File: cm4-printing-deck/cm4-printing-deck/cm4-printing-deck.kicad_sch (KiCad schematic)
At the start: 200 parts, among them J1 Micro_SD_Card, J10 KB_USB, J2 USB_C_Receptacle_USB2.0_14P, J3 Reset, J4 debug, J5 Boot pins, J6 HDMI_A, J7 USB3_A, J8 USB3_A, J9 KB_USB, K1 KEYSW, K10 KEYSW, K11 KEYSW, K12 KEYSW, K13 KEYSW, K14 KEYSW, K15 KEYSW, K16 KEYSW, K17 KEYSW, K18 KEYSW, K19 KEYSW, K2 KEYSW, K20 KEYSW, K21 KEYSW, K22 KEYSW, K23 KEYSW, K24 KEYSW, K25 KEYSW, K26 KEYSW, K27 KEYSW, K28 KEYSW, K29 KEYSW, K3 KEYSW, K30 KEYSW, K31 KEYSW, K32 KEYSW, K33 KEYSW, K34 KEYSW, K35 KEYSW, K36 KEYSW, K37 KEYSW, K38 KEYSW, K39 KEYSW, K4 KEYSW, K40 KEYSW, K41 KEYSW, K42 KEYSW, K43 KEYSW, K44 KEYSW, K45 KEYSW, K46 KEYSW, K47 KEYSW, K48 KEYSW, K49 KEYSW, K5 KEYSW, K50 KEYSW, K51 KEYSW, K52 KEYSW, K53 KEYSW, K54 KEYSW, K55 KEYSW, K56 KEYSW, K57 KEYSW, K6 KEYSW, K60 KEYSW, K61 KEYSW, K7 KEYSW, K8 KEYSW, K9 KEYSW, SW20 Power, SW62 WIFIBT_DISABLE, U1 Compute_Module_4_Connectors, U10 AP2112K-3.3, U11 W25Q128JVS, U2 RP2040, U3 RT9742GGJ5, U5 PCF85063ATL, U6 74LVC1G07, U7 74LVC1G07, U8 74LVC1G07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

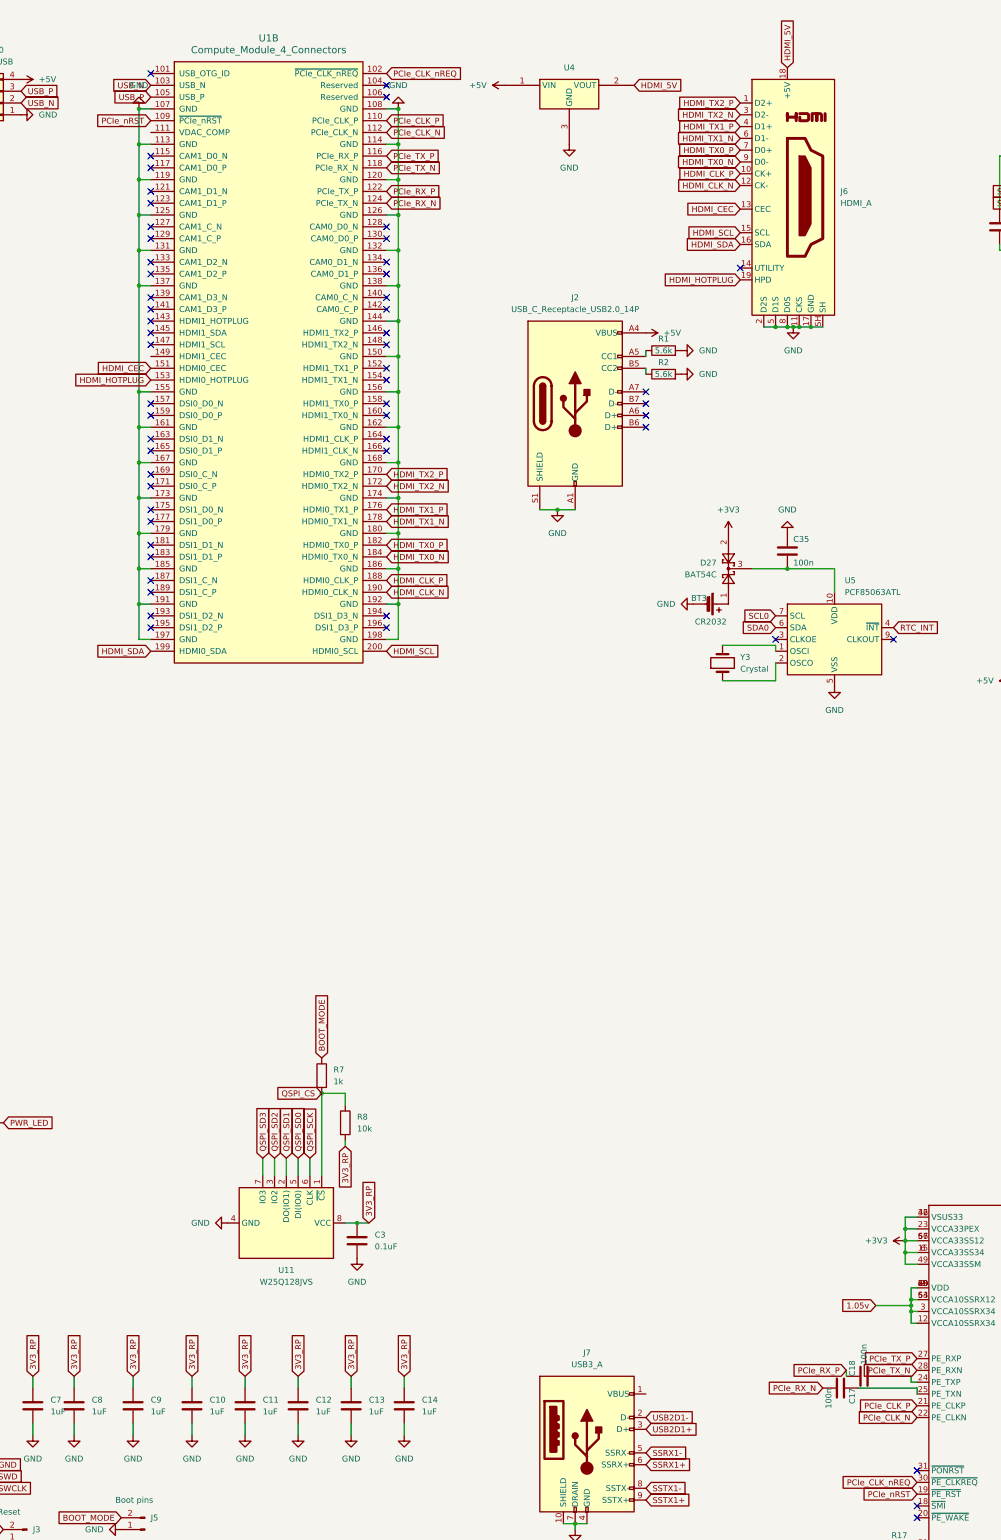
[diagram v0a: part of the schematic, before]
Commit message: minor routing and placement changes
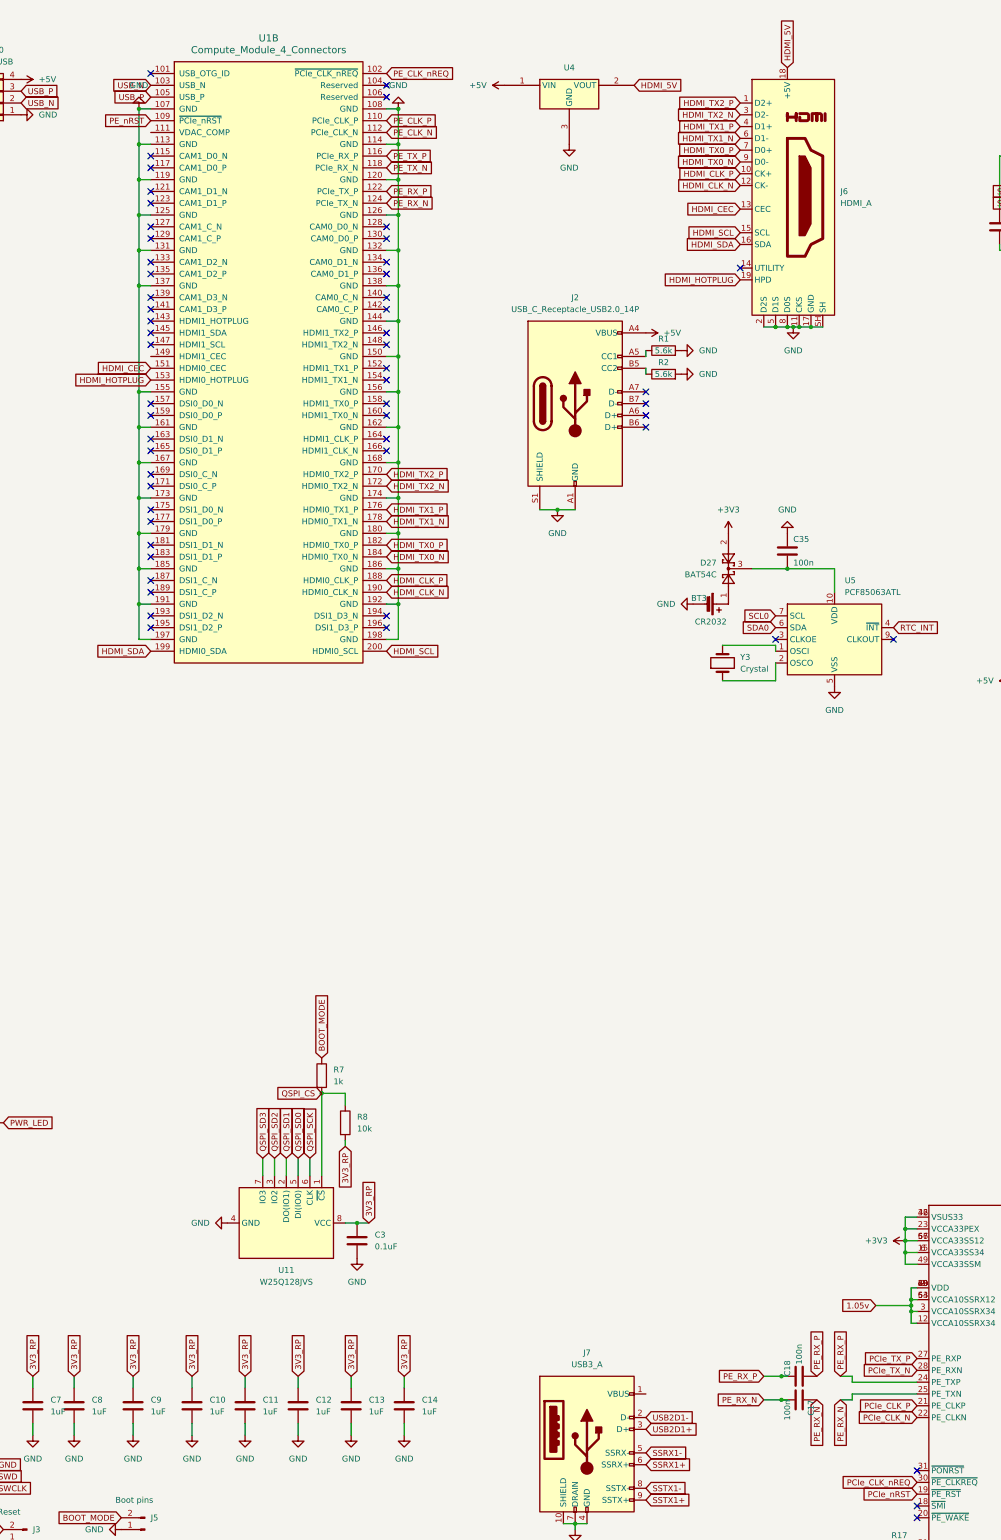
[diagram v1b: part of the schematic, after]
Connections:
- net PCIe_RX_N is gone; now on net PE_RX_N: C17.1, U1.124 (PCIe_TX_N)
- net PCIe_RX_P is gone; now on net PE_RX_P: C18.1, U1.122 (PCIe_TX_P)
- net PCIe_CLK_N: no longer U1.112 (PCIe_CLK_N)
- net PCIe_CLK_P: no longer U1.110 (PCIe_CLK_P)
- net PCIe_CLK_nREQ: no longer U1.102 (~{PCIe_CLK_nREQ})
- net PCIe_TX_N: no longer U1.118 (PCIe_RX_N)
- net PCIe_TX_P: no longer U1.116 (PCIe_RX_P)
- net PCIe_nRST: no longer U1.109 (~{PCIe_nRST})
- net PE_RX_P: now reaches C18.2, U9.24 (PE_TXP)
- net PE_RX_N: now reaches C17.2, U9.25 (PE_TXN)
- new net PE_CLK_N: U1.112 (PCIe_CLK_N)
- new net PE_CLK_P: U1.110 (PCIe_CLK_P)
- new net PE_CLK_nREQ: U1.102 (~{PCIe_CLK_nREQ})
- new net PE_TX_N: U1.118 (PCIe_RX_N)
- new net PE_TX_P: U1.116 (PCIe_RX_P)
- new net PE_nRST: U1.109 (~{PCIe_nRST})
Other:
- moved on the sheet: C17, C18

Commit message: cm4-printing-deck: added fpc connectors for dsi panel
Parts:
- added C19, C20, C21: 0.1uF 10V, Capacitor_SMD:C_0402_1005Metric, symbol Device:C
- added C22: 22uF 6.3V, Capacitor_SMD:C_0402_1005Metric, symbol Device:C
- added C23, C24, C25, C27: 0.1uF 6.3V, Capacitor_SMD:C_0402_1005Metric, symbol Device:C
- added C26: 0.1uF 6V3, Capacitor_SMD:C_0603_1608Metric, symbol Device:C
- added C4: 22uF 10V, Capacitor_SMD:C_0402_1005Metric, symbol Device:C
- added J11: 3-2328724-1, moth:3-2328724-1, symbol cm4-panel-jdi-lt070me05000-rescue:3-2328724-1-Connector
- added J12: MOLEX_503480-0600, moth:screen_conn_2_nexus, symbol cm4-panel-jdi-lt070me05000-rescue:503480-0600-503480-0600
- added L1: BLM18TG121TN1D, Inductor_SMD:L_0603_1608Metric, symbol Device:L
- added R10, R19, R20, R21, R9: 10k 5%, Resistor_SMD:R_0402_1005Metric, symbol Device:R
- added U12: SN74LVC1G34DBVRG4, Package_TO_SOT_SMD:SOT-23-5, symbol cm4-panel-jdi-lt070me05000-rescue:SN74LVC1G34DBVRG4-Logic_LevelTranslator
- added U13: MCP23008T-E_SS, Package_SO:SSOP-20_5.3x7.2mm_P0.65mm, symbol cm4-panel-jdi-lt070me05000-rescue:MCP23008T-E_SS-MCP23008T-E_SS
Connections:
- net +3V3: now also C22.2, C23.2, C26.2, J11.26 (VDDp), J11.27 (VDDp), L1.2, R20.1, R21.1, U13.20 (VDD)
- net +5V: now also C19.2, C20.2, C21.2, C4.2, J11.1 (VDD), J11.2 (VDD), J11.3 (VDD), J11.4 (VDD)
- net GND: now also C19.1, C20.1, C21.1, C22.1, C23.1, C24.1, C25.1, C26.1, C27.1, C4.1, J11.11 (GND), J11.14 (GND), J11.17 (GND), J11.20 (GND), J11.23 (GND), J11.28 (GND), J11.29 (GND), J11.5 (GND), J11.8 (GND), J11.SH, J12.4, J12.S1 (SHIELD), J12.S2 (SHIELD), R10.2, R19.2, R9.1, U12.1 (NC), U12.3 (GND), U13.3 (A2), U13.4 (A1), U13.5 (A0), U13.9 (VSS)
- net SCL0: no longer U1.80 (I2C_SCL0)
- net SDA0: no longer U1.82 (I2C_SDA0)
- net MIPI_0_N: now reaches U1.175 (DSI1_D0_N)
- net MIPI_0_N: now also J11.12 (MIPI_0N)
- net MIPI_0_P: now reaches U1.177 (DSI1_D0_P)
- net MIPI_0_P: now also J11.13 (MIPI_0P)
- net MIPI_1_N: now reaches U1.181 (DSI1_D1_N)
- net MIPI_1_N: now also J11.18 (MIPI_1N)
- net MIPI_1_P: now reaches U1.183 (DSI1_D1_P)
- net MIPI_1_P: now also J11.19 (MIPI_1P)
- net MIPI_CLK_N: now reaches U1.187 (DSI1_C_N)
- net MIPI_CLK_N: now also J11.15 (MIPI_CLKN)
- net MIPI_CLK_P: now reaches U1.189 (DSI1_C_P)
- net MIPI_CLK_P: now also J11.16 (MIPI_CLKP)
- net MIPI_2_N: now reaches U1.193 (DSI1_D2_N)
- net MIPI_2_N: now also J11.21 (MIPI_2N)
- net MIPI_3_N: now reaches U1.194 (DSI1_D3_N)
- net MIPI_3_N: now also J11.9 (MIPI_3N)
- net MIPI_2_P: now reaches U1.195 (DSI1_D2_P)
- net MIPI_2_P: now also J11.22 (MIPI_2P)
- net MIPI_3_P: now reaches U1.196 (DSI1_D3_P)
- net MIPI_3_P: now also J11.10 (MIPI_3P)
- new net: R20.2, U13.6 (*RESET)
- new net: C27.2, J12.1, L1.1
- new net: J11.24 (XRES), U12.4 (Y)
- new net +1V8: C24.2, C25.2, J11.31 (IOVCC), U12.5 (VCC)
- new net BL_CNTRL: J11.6 (LED_EN), R10.1, U13.16 (GP4)
- new net EXP_INT: R21.2, U13.8 (INT)
- new net EXP_P2: U13.14 (GP2)
- new net LCD_PWR_EN: J11.30 (DCDC_EN), R9.2, U13.17 (GP5)
- new net LCD_RESET: R19.1, U12.2 (A), U13.15 (GP3)
- new net SCL: J12.6, U1.80 (I2C_SCL0), U13.1 (SCL)
- new net SDA: J12.5, U1.82 (I2C_SDA0), U13.2 (SDA)
- new net TOUCH_INT: J12.2, U13.13 (GP1)
- new net TOUCH_RST: J12.3, U13.12 (GP0)
- no-connect marks 138 -> 136
